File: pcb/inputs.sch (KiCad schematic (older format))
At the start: 61 parts, among them U11 MPXA6115AC6U, U4 MAX9926UAEE+, U6 MPX4250AP

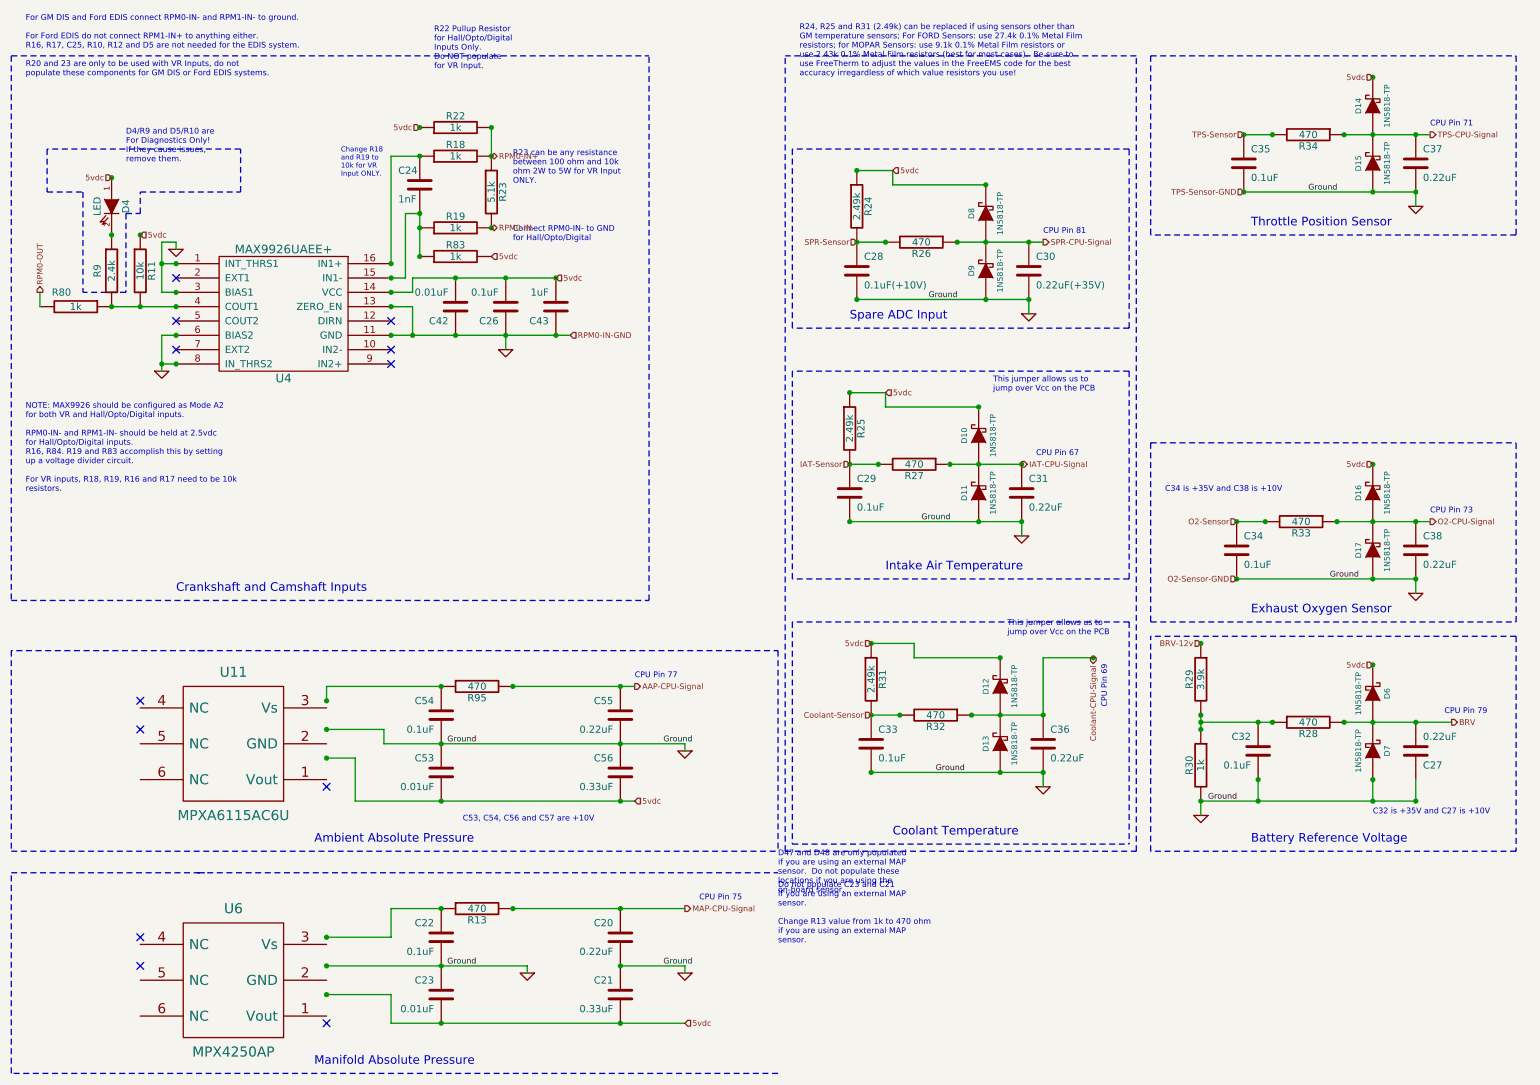
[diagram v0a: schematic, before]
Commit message: MPX4250 footprint
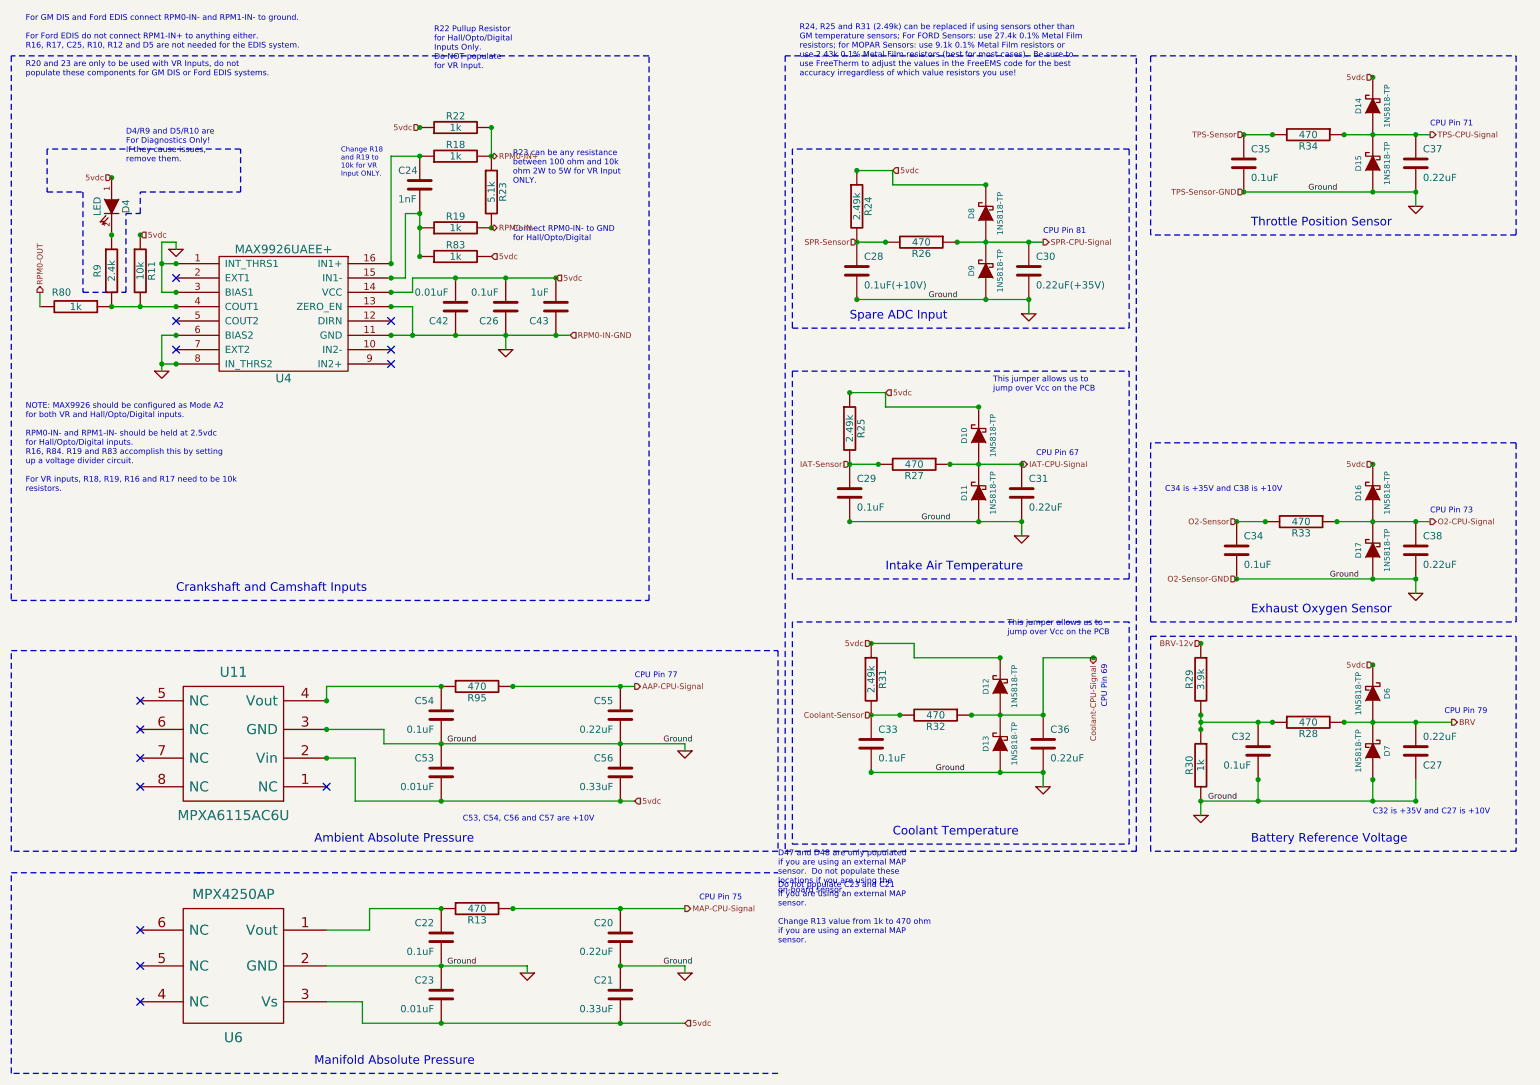
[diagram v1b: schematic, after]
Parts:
- removed U11: MPXA6115AC6U, symbol MPXA4250AP
- added U11: MPXA6115AC6U, ~, symbol MPXA6115AC6U
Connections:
- net 5vdc: now also U6.3 (Vs), U11.2 (Vin)
- net GND: now also U6.2 (GND), U11.3 (GND)
- net at C22.1, R13.1: now also U6.1 (Vout)
- net at C54.1, R95.1: now also U11.4 (Vout)
- no-connect marks 12 -> 14
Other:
- moved on the sheet: U6
